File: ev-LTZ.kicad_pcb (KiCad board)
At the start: 2 copper layers, 50 x 100 mm, 41 parts, among them P1 VIN+, P2 CONN_01X02, P3 VH-, P4 VH+, P5 SENSE-, P6 SENSE+, P7 VIN-, Q1 BD139, U1 LT1013N8

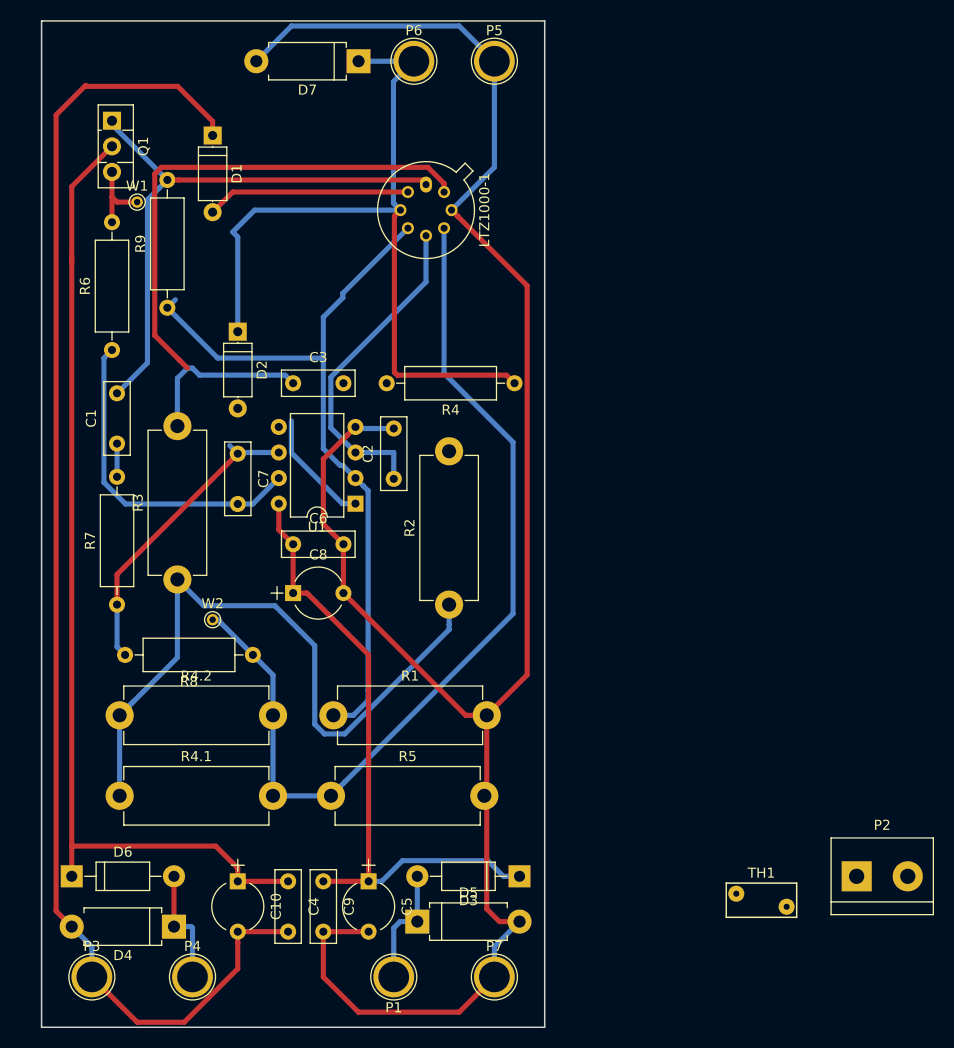
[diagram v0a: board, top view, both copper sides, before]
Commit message: pcb
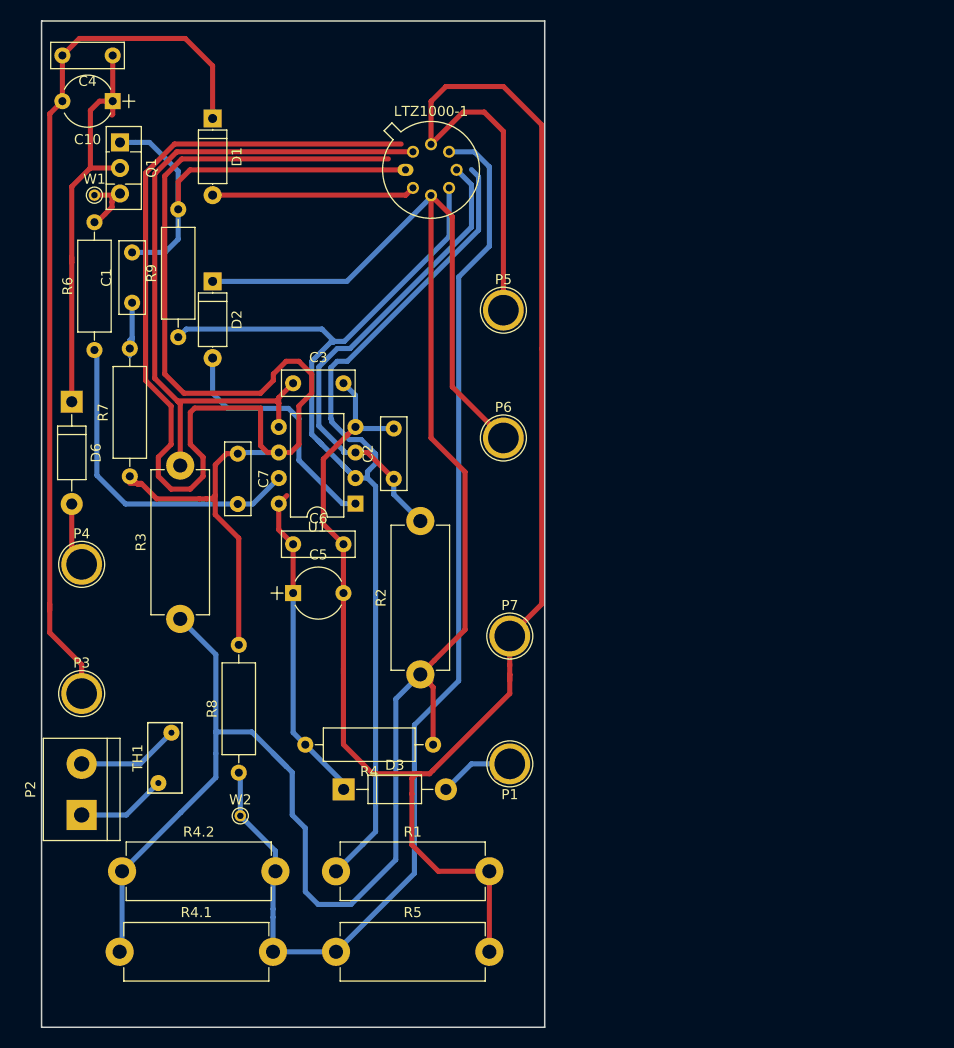
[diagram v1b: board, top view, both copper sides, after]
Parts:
- removed C8: 1uF, Capacitors_THT:CP_Radial_Tantal_D5.0mm_P5.00mm
- removed C9: .1uF, Capacitors_THT:C_Rect_L7.2mm_W2.5mm_P5.00mm_FKS2_FKP2_MKS2_MKP2
- removed D4, D5, D7: D_TVS, Diodes_THT:D_DO-15_P10.16mm_Horizontal
- C10, C5: value 1uF -> 47uF
- moved C4 83.9 mm to (137.1, 53.4), turned to 180 degrees
- moved C10 78.5 mm to (137.1, 58.0), turned to 180 degrees
- moved P2 77.3 mm to (134.0, 128.9), turned to 90 degrees
- moved TH1 63.5 mm to (142.9, 120.7), turned to 270 degrees
- moved D6 47.2 mm to (133.0, 87.8), turned to 270 degrees
- moved P4 42.5 mm to (134.0, 104.0)
- moved P6 38.5 mm to (175.9, 91.4)
- moved R4 36.8 mm to (168.9, 121.9)
- moved P7 33.9 mm to (176.5, 111.1)
- moved C5 29.6 mm to (155.0, 106.9), turned to 0 degrees
- moved P3 28.2 mm to (134.0, 116.8)
- moved P5 24.8 mm to (175.9, 78.7)
- moved P1 24.1 mm to (176.5, 123.8)
- moved W2 19.7 mm to (149.8, 129.0)
- moved D3 19.5 mm to (160.0, 126.4), turned to 0 degrees
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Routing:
- net Net-(C7-Pad1): track 30.6 -> 190.2 mm
- net Net-(LTZ1000-1-Pad4): track 75.2 -> 138.4 mm
- net Net-(C10-Pad1): track 98.5 -> 41.0 mm
- net /SENSE+: track 148.4 -> 203.9 mm
- net /VH-: track 134.0 -> 87.9 mm
- net Net-(C5-Pad1): track 63.0 -> 32.2 mm
- net /TSENSE: track 92.8 -> 114.6 mm
- net Net-(C2-Pad1): track 32.9 -> 48.1 mm
- net Net-(D2-Pad2): track 11.6 -> 24.6 mm
- net Net-(C1-Pad2): track 57.6 -> 44.7 mm
- net Net-(P2-Pad2): track 0.11 -> 10.2 mm
- net Net-(P2-Pad1): track 0.11 -> 8.94 mm
- net GND: track 198.4 -> 191.5 mm
- net /VH+: track 11.8 -> 6.62 mm
- net Net-(C3-Pad1): track 68.5 -> 71.8 mm
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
